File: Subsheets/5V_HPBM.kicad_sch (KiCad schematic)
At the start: 8 parts, among them Q1 BSS123NH6327XTSA1

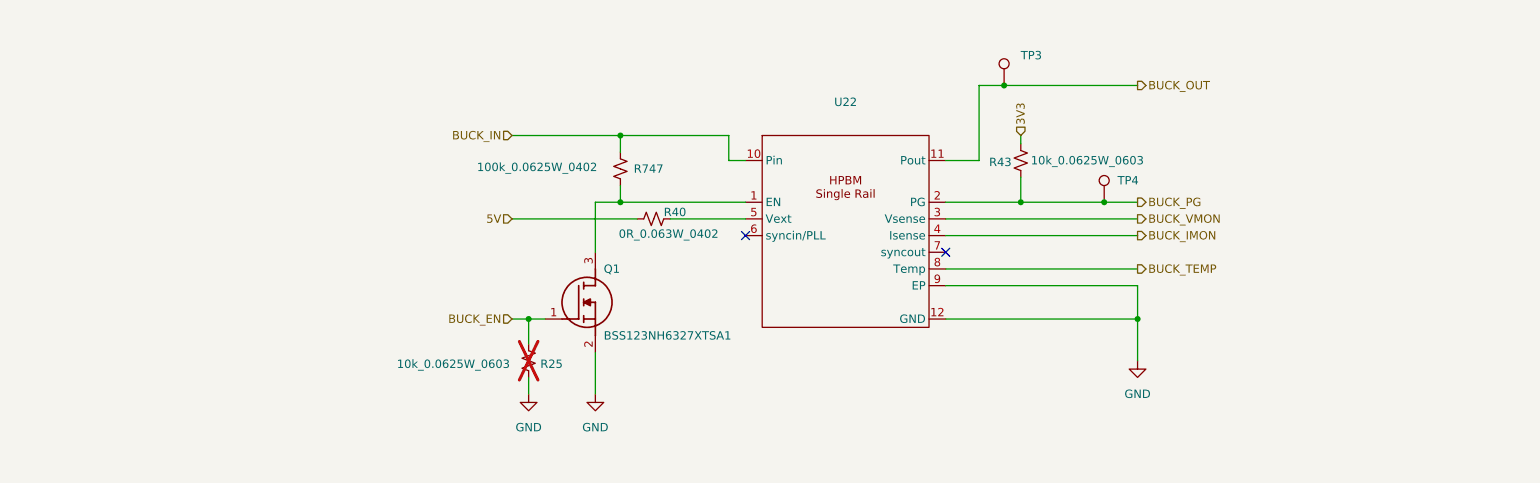
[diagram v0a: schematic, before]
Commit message: Schematic Update 1.2
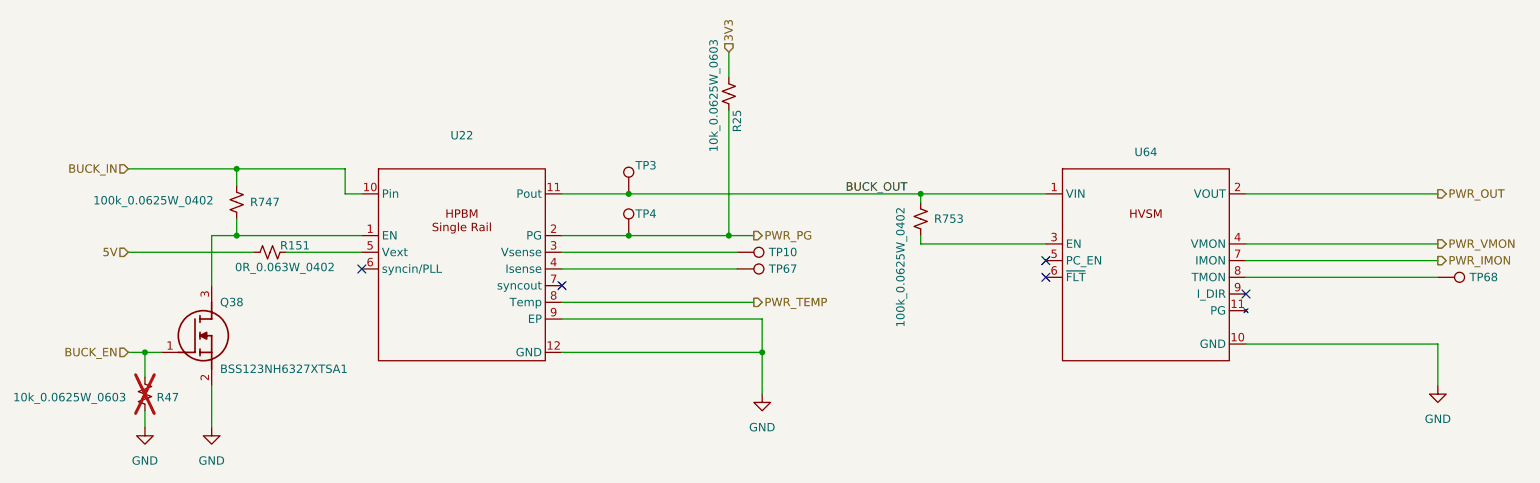
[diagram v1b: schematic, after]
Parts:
- removed Q1: BSS123NH6327XTSA1, SOT95P240X110-3N, symbol BSS123NH6327XTSA1:BSS123NH6327XTSA1
- removed R40: 0R_0.063W_0402, Pixxel_Resistors:RES0402, symbol Device:R_Small_US
- removed R43: 10k_0.0625W_0603, Pixxel_Resistors:RES0603, symbol Device:R_Small_US
- added Q38: BSS123NH6327XTSA1, SOT95P240X110-3N, symbol BSS123NH6327XTSA1:BSS123NH6327XTSA1
- added R151: 0R_0.063W_0402, Pixxel_Resistors:RES0402, symbol Device:R_Small_US
- added R47: 10k_0.0625W_0603, Pixxel_Resistors:RES0603, symbol Device:R_Small_US
- added R753: 100k_0.0625W_0402, Pixxel_Resistors:RES0402, symbol Device:R_Small_US
- added TP10, TP67, TP68: TestPoint, symbol Connector:TestPoint
- added U64: (no value), symbol HVSM_LVSM_v9:HVSM
- R25: now fitted
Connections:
- net 3V3: now also R25.1
- net 5V: now also R151.2
- net BUCK_EN: now also Q38.1 (G), R47.1; no longer R25.1
- net BUCK_OUT: now also R753.2, U64.1 (VIN)
- net GND: now also Q38.2 (S), R47.2, U64.10 (GND); no longer R25.2
- net at U22.5 (Vext): now also R151.1
- net at R747.1, U22.1 (EN): now also Q38.3 (D)
- net BUCK_IMON: no longer names the net of U22.4 (Isense)
- net BUCK_IMON: now also TP67.1
- net BUCK_PG renamed PWR_PG
- net PWR_PG: now also R25.2
- net BUCK_TEMP renamed PWR_TEMP
- net BUCK_VMON: no longer names the net of U22.3 (Vsense)
- net BUCK_VMON: now also TP10.1
- new net: R753.1, U64.3 (EN)
- new net: TP68.1, U64.8 (TMON)
- new net PWR_IMON: U64.7 (IMON)
- new net PWR_OUT: U64.2 (VOUT)
- new net PWR_VMON: U64.4 (VMON)
- no-connect marks 2 -> 5
